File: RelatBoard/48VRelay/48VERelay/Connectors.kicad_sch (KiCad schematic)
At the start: 3 parts, among them J2 RJ45_Hanrun_HR911105A_Horizon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

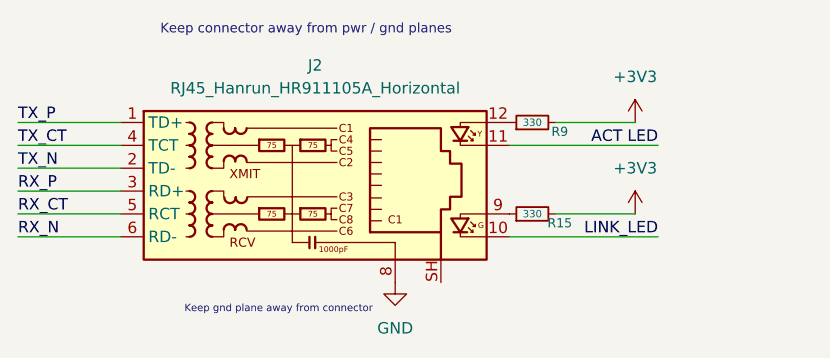
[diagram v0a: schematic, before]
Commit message: begin pcb design
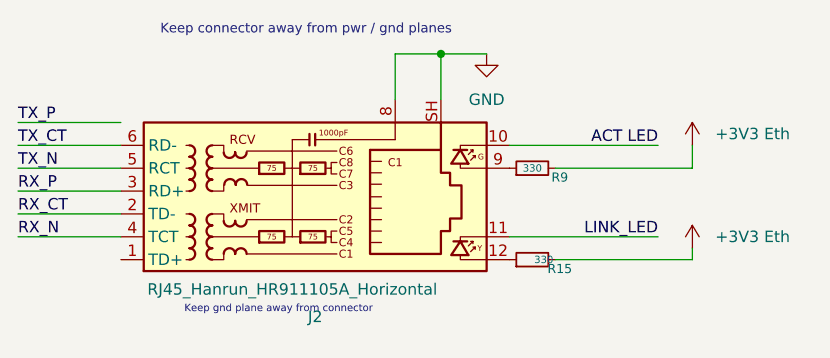
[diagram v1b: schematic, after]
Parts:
- R15, R9: footprint (none) -> Resistor_SMD:R_0603_1608Metric
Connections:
- net ACT LED: now also J2.10; no longer J2.11
- net GND: now also J2.SH
- net LINK_LED: now also J2.11; no longer J2.10
- net RX_CT: now also J2.2 (TD-); no longer J2.5 (RCT)
- net RX_N: now also J2.4 (TCT); no longer J2.6 (RD-)
- net TX_CT: now also J2.6 (RD-); no longer J2.4 (TCT)
- net TX_N: now also J2.5 (RCT); no longer J2.2 (TD-)
- net TX_P: no longer J2.1 (TD+)
- net at R15.1: now also J2.12; no longer J2.9
- net at R9.1: now also J2.9; no longer J2.12
- net +3V3 renamed +3V3 Eth
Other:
- moved on the sheet: J2, R15, R9
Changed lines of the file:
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@@
 		)
 	)
-	(wire
-		(pts
-			(xy 231.14 48.26) (xy 222.25 48.26)
+	(junction
+		(at 209.55 40.64)
+		(diameter 0)
+		(color 0 0 0 0)
+	)
+	(wire
+		(pts
+			(xy 209.55 45.72) (xy 209.55 40.64)
+		)
+		(stroke
+			(width 0)
+			(type default)
+		)
+	)
+	(wire
+		(pts
+			(xy 222.25 53.34) (xy 237.49 53.34)
 		)
 		(stroke
@@
 	(wire
 		(pts
+			(xy 237.49 63.5) (xy 237.49 62.23)
+		)
+		(stroke
+			(width 0)
+			(type default)
+		)
+	)
+	(wire
+		(pts
 			(xy 162.56 55.88) (xy 173.99 55.88)
 		)
@@
 	(wire
 		(pts
+			(xy 204.47 45.72) (xy 204.47 40.64)
+		)
+		(stroke
+			(width 0)
+			(type default)
+		)
+	)
+	(wire
+		(pts
+			(xy 204.47 40.64) (xy 209.55 40.64)
+		)
+		(stroke
+			(width 0)
+			(type default)
+		)
+	)
+	(wire
+		(pts
 			(xy 162.56 60.96) (xy 173.99 60.96)
 		)
@@
 	(wire
 		(pts
-			(xy 231.14 58.42) (xy 222.25 58.42)
+			(xy 222.25 63.5) (xy 237.49 63.5)
+		)
+		(stroke
+			(width 0)
+			(type default)
+		)
+	)
+	(wire
+		(pts
+			(xy 209.55 40.64) (xy 214.63 40.64)
 		)
 		(stroke
@@
 		(pts
 			(xy 173.99 53.34) (xy 162.56 53.34)
+		)
+		(stroke
+			(width 0)
+			(type default)
+		)
+	)
+	(wire
+		(pts
+			(xy 237.49 53.34) (xy 237.49 50.8)
 		)
 		(stroke
@@
 	(symbol
 		(lib_id "Device:R_Small")
-		(at 219.71 58.42 90)
+		(at 219.71 63.5 90)
 		(unit 1)
 		(body_style 1)
@@
 		(dnp no)
 		(property "Reference" "R15"
-			(at 222.758 59.436 90)
+			(at 222.758 64.516 90)
 			(show_name no)
 			(do_not_autoplace no)
@@
 		)
 		(property "Value" "330"
-			(at 219.71 58.42 90)
+			(at 220.98 63.5 90)
 			(show_name no)
 			(do_not_autoplace no)
@@
 			)
 		)
-		(property "Footprint" ""
-			(at 219.71 58.42 0)
+		(property "Footprint" "Resistor_SMD:R_0603_1608Metric"
+			(at 219.71 63.5 0)
 			(hide yes)
 			(show_name no)
@@
 		)
 		(property "Datasheet" ""
-			(at 219.71 58.42 0)
+			(at 219.71 63.5 0)
 			(hide yes)
 			(show_name no)
@@
 		)
 		(property "Description" "Resistor, small symbol"
-			(at 219.71 58.42 0)
+			(at 219.71 63.5 0)
 			(hide yes)
 			(show_name no)
@@
 	(symbol
 		(lib_id "power:+3V3")
-		(at 231.14 58.42 0)
+		(at 237.49 62.23 0)
 		(mirror y)
 		(unit 1)
@@
 		(fields_autoplaced yes)
 		(property "Reference" "#PWR031"
-			(at 231.14 62.23 0)
-			(hide yes)
-			(show_name no)
-			(do_not_autoplace no)
-			(effects
-				(font
-					(size 1.27 1.27)
-				)
-			)
-		)
-		(property "Value" "+3V3"
-			(at 231.14 53.34 0)
-			(show_name no)
-			(do_not_autoplace no)
-			(effects
-				(font
-					(size 1.27 1.27)
-				)
+			(at 237.49 66.04 0)
+			(hide yes)
+			(show_name no)
+			(do_not_autoplace no)
+			(effects
+				(font
+					(size 1.27 1.27)
+				)
+			)
+		)
+		(property "Value" "+3V3 Eth"
+			(at 240.03 60.9599 0)
+			(show_name no)
+			(do_not_autoplace no)
+			(effects
+				(font
+					(size 1.27 1.27)
+				)
+				(justify right)
 			)
 		)
 		(property "Footprint" ""
-			(at 231.14 58.42 0)
+			(at 237.49 62.23 0)
 			(hide yes)
 			(show_name no)
@@
 		)
 		(property "Datasheet" ""
-			(at 231.14 58.42 0)
+			(at 237.49 62.23 0)
 			(hide yes)
 			(show_name no)
@@
 		)
 		(property "Description" "Power symbol creates a global label with name \"+3V3\""
-			(at 231.14 58.42 0)
+			(at 237.49 62.23 0)
 			(hide yes)
 			(show_name no)
@@
 	(symbol
 		(lib_id "power:+3V3")
-		(at 231.14 48.26 0)
+		(at 237.49 50.8 0)
 		(mirror y)
 		(unit 1)
@@
 		(fields_autoplaced yes)
 		(property "Reference" "#PWR030"
-			(at 231.14 52.07 0)
-			(hide yes)
-			(show_name no)
-			(do_not_autoplace no)
-			(effects
-				(font
-					(size 1.27 1.27)
-				)
-			)
-		)
-		(property "Value" "+3V3"
-			(at 231.14 43.18 0)
-			(show_name no)
-			(do_not_autoplace no)
-			(effects
-				(font
-					(size 1.27 1.27)
-				)
+			(at 237.49 54.61 0)
+			(hide yes)
+			(show_name no)
+			(do_not_autoplace no)
+			(effects
+				(font
+					(size 1.27 1.27)
+				)
+			)
+		)
+		(property "Value" "+3V3 Eth"
+			(at 240.03 49.5299 0)
+			(show_name no)
+			(do_not_autoplace no)
+			(effects
+				(font
+					(size 1.27 1.27)
+				)
+				(justify right)
 			)
 		)
 		(property "Footprint" ""
-			(at 231.14 48.26 0)
+			(at 237.49 50.8 0)
 			(hide yes)
 			(show_name no)
@@
 		)
 		(property "Datasheet" ""
-			(at 231.14 48.26 0)
+			(at 237.49 50.8 0)
 			(hide yes)
 			(show_name no)
@@
 		)
 		(property "Description" "Power symbol creates a global label with name \"+3V3\""
-			(at 231.14 48.26 0)
+			(at 237.49 50.8 0)
 			(hide yes)
 			(show_name no)
@@
 		(lib_id "Connector:RJ45_Hanrun_HR911105A_Horizontal")
 		(at 194.31 55.88 0)
+		(mirror x)
 		(unit 1)
 		(body_style 1)
-		(exclude_from_sim no)
+		(exclude_from_sim yes)
 		(in_bom yes)
 		(on_board yes)
 		(in_pos_files yes)
 		(dnp no)
-		(fields_autoplaced yes)
 		(property "Reference" "J2"
-			(at 195.58 41.91 0)
+			(at 195.58 69.85 0)
 			(show_name no)
 			(do_not_autoplace no)
@@
 		)
 		(property "Value" "RJ45_Hanrun_HR911105A_Horizontal"
-			(at 195.58 44.45 0)
+			(at 193.04 66.802 0)
 			(show_name no)
 			(do_not_autoplace no)
@@
 		)
 		(property "Footprint" "Connector_RJ:RJ45_Hanrun_HR911105A_Horizontal"
-			(at 194.31 43.18 0)
+			(at 194.31 68.58 0)
 			(hide yes)
 			(show_name no)
@@
 		)
 		(property "Datasheet" "https://datasheet.lcsc.com/lcsc/1811141815_HANRUN-Zhongshan-HanRun-Elec-HR911105A_C12074.pdf"
-			(at 194.31 40.64 0)
+			(at 194.31 71.12 0)
 			(hide yes)
 			(show_name no)
@@
 	(symbol
 		(lib_id "power:GND")
-		(at 204.47 66.04 0)
+		(at 214.63 40.64 0)
 		(unit 1)
 		(body_style 1)
@@
 		(fields_autoplaced yes)
 		(property "Reference" "#PWR018"
-			(at 204.47 72.39 0)
+			(at 214.63 46.99 0)
 			(hide yes)
 			(show_name no)
@@
 		)
 		(property "Value" "GND"
-			(at 204.47 71.12 0)
+			(at 214.63 45.72 0)
 			(show_name no)
 			(do_not_autoplace no)
@@
 		)
 		(property "Footprint" ""
-			(at 204.47 66.04 0)
+			(at 214.63 40.64 0)
 			(hide yes)
 			(show_name no)
@@
 		)
 		(property "Datasheet" ""
-			(at 204.47 66.04 0)
+			(at 214.63 40.64 0)
 			(hide yes)
 			(show_name no)
@@
 		)
 		(property "Description" "Power symbol creates a global label with name \"GND\" , ground"
-			(at 204.47 66.04 0)
+			(at 214.63 40.64 0)
 			(hide yes)
 			(show_name no)
@@
 	(symbol
 		(lib_id "Device:R_Small")
-		(at 219.71 48.26 90)
+		(at 219.71 53.34 90)
 		(unit 1)
 		(body_style 1)
@@
 		(dnp no)
 		(property "Reference" "R9"
-			(at 222.758 49.276 90)
+			(at 222.758 54.356 90)
 			(show_name no)
 			(do_not_autoplace no)
@@
 		)
 		(property "Value" "330"
-			(at 219.71 48.26 90)
+			(at 219.71 53.34 90)
 			(show_name no)
 			(do_not_autoplace no)
@@
 			)
 		)
-		(property "Footprint" ""
-			(at 219.71 48.26 0)
+		(property "Footprint" "Resistor_SMD:R_0603_1608Metric"
+			(at 219.71 53.34 0)
 			(hide yes)
 			(show_name no)
@@
 		)
 		(property "Datasheet" ""
-			(at 219.71 48.26 0)
+			(at 219.71 53.34 0)
 			(hide yes)
 			(show_name no)
@@
 		)
 		(property "Description" "Resistor, small symbol"
-			(at 219.71 48.26 0)
-			(hide yes)
-			(show_name no)
+			(at 219.71 53.34 0)
+			(hide yes)
+			(show_name no)
